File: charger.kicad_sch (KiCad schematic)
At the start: 37 parts, among them Q1 NMOS, Q2 NMOS, U2 BQ25798RQMR

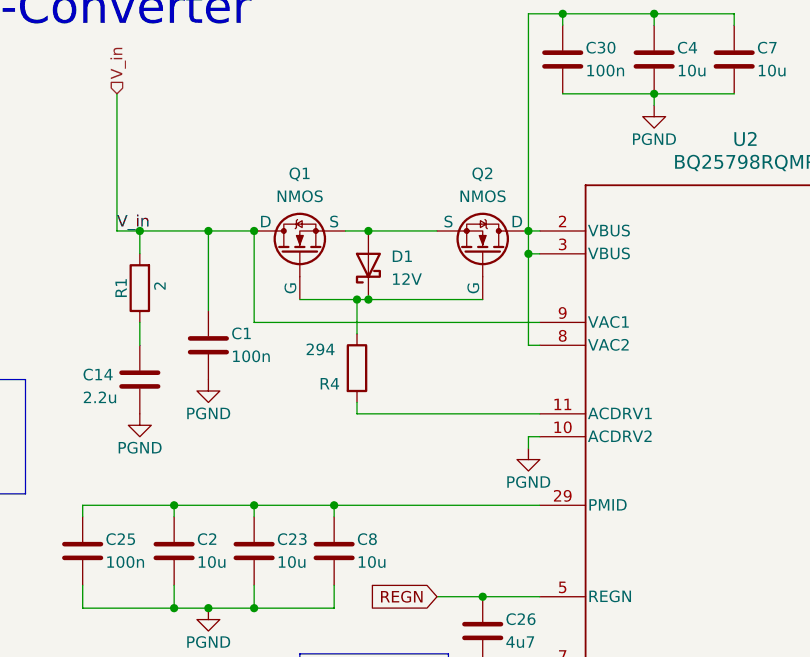
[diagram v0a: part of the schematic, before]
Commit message: started routing Please enter the commit message for your changes. Lines starting
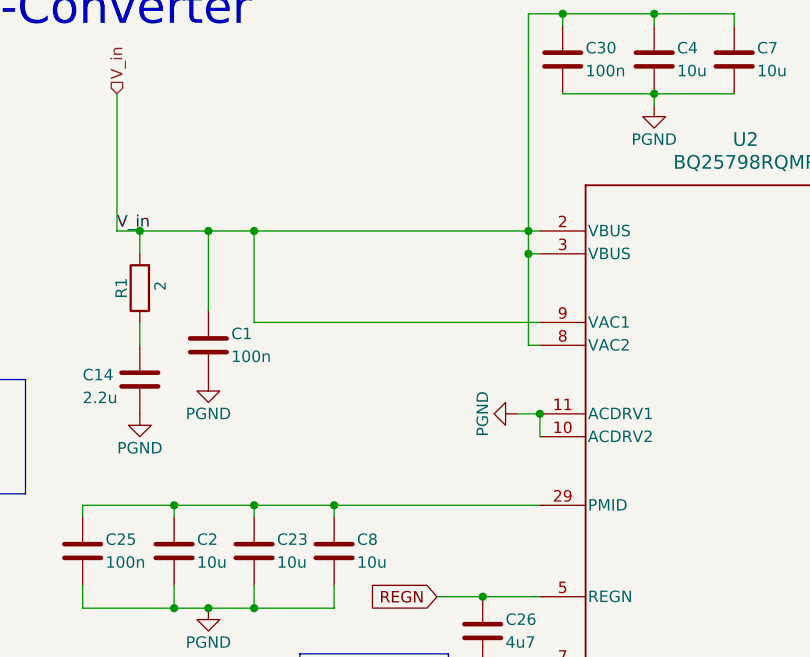
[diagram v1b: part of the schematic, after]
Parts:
- removed D1: 12V, Diode_SMD:D_SOD-523, symbol Device:D_Schottky
- removed Q1, Q2: NMOS, Package_TO_SOT_THT:TO-220-3_Horizontal_TabDown, symbol Simulation_SPICE:NMOS
- removed R4: 294, Resistor_SMD:R_0603_1608Metric, symbol Device:R
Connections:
- net PGND: now also U2.11 (ACDRV1)
- net V_in: now also C30.1, C4.1, C7.1, U2.2 (VBUS), U2.3 (VBUS), U2.8 (VAC2)
